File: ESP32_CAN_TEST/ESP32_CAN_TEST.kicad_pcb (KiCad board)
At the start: 2 copper layers, 45.7 x 45.7 mm, 34 parts, among them J1 5V in, J2 Encoder_1, J3 Molex_2x2, J4 Encoder2, J5 i2C, J6 UART, J7 GH1.25, J8 JST_2.54, Q1 2N7002, Q2 2N7002, SW1 EN, SW2 EN, U1 AMS1117, U2 ESP32-WROOM-32, U3 TJA1050

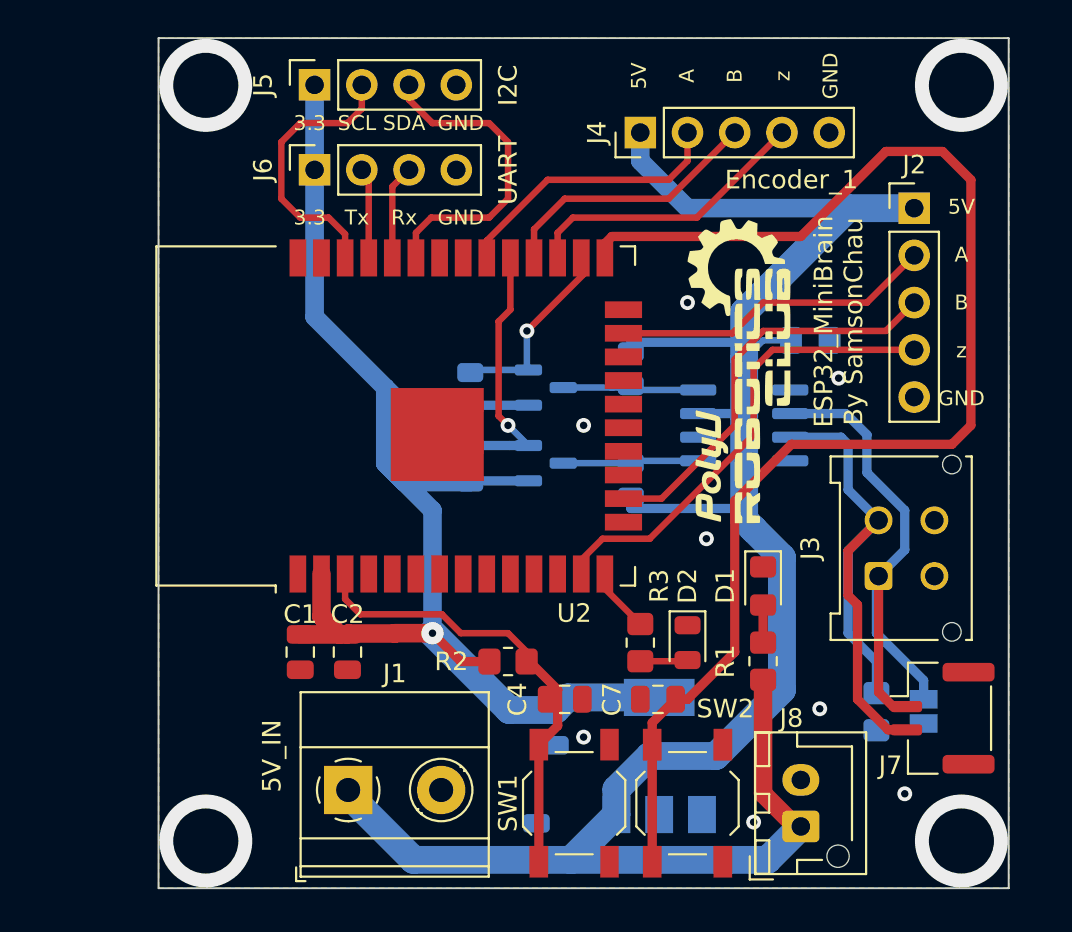
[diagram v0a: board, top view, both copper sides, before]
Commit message: ESP,Power board update
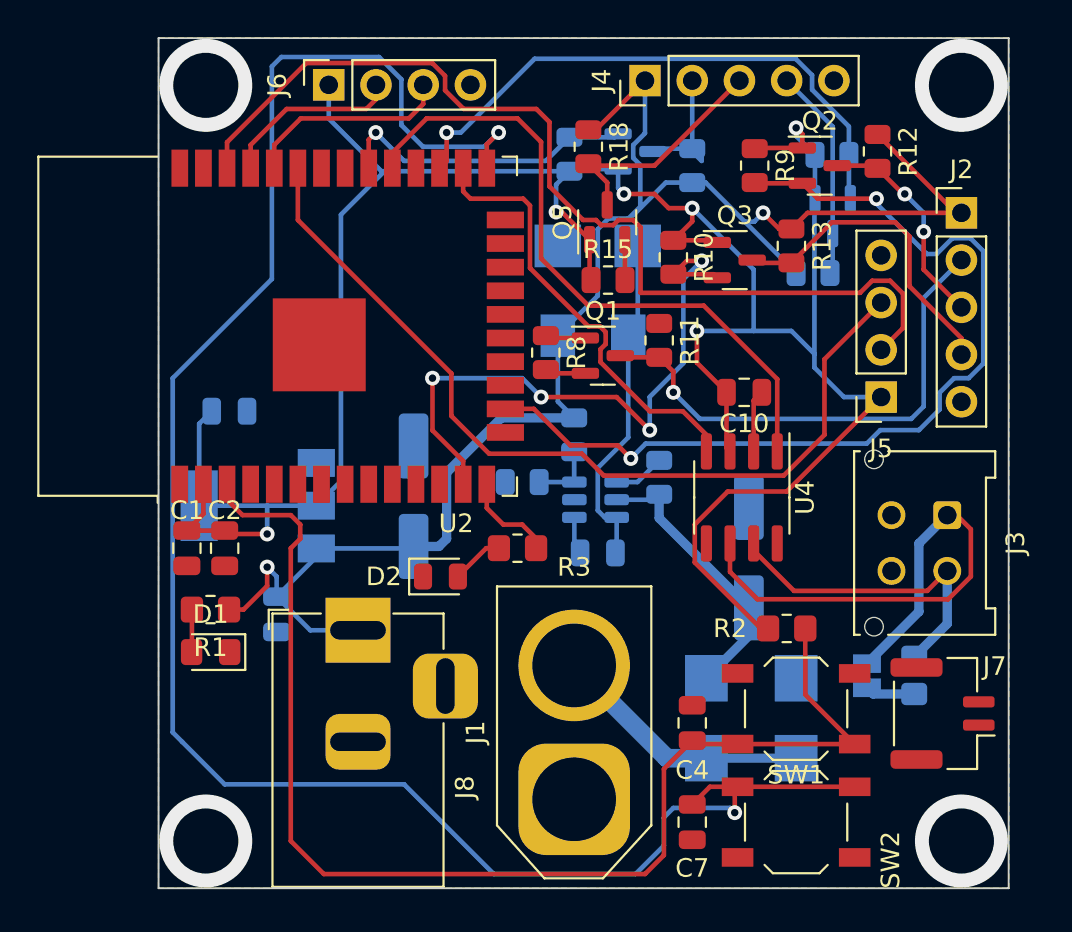
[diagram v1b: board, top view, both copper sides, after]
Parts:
- removed G***: LOGO, PolyuRobotics:Club_logo
- added C10: 0.1u, Capacitor_SMD:C_0805_2012Metric, F.Cu at (133.1, 59.7)
- added C8: 100nF, Capacitor_SMD:C_0805_2012Metric, B.Cu at (125.2, 68.3)
- added C9: 16V 22UF, Capacitor_SMD:CP_Elec_6.3x7.7, B.Cu at (115.3, 65.3)
- added D3: SMBJ24CA, Diode_SMD:D_SMB, B.Cu at (135.9, 77.2)
- added D4: SS34, Diode_SMD:D_SMB, B.Cu at (131.1, 77.2)
- added D5: SS34, Diode_SMD:D_SMB, B.Cu at (125.2, 51.8)
- added L1: 22uH, Inductor_SMD:L_Vishay_IHLP-1616, B.Cu at (125.0, 56.6)
- added Q3: 2N7002, Package_TO_SOT_SMD:SOT-23, F.Cu at (132.6, 52.6)
- added Q4: 2N7002, Package_TO_SOT_SMD:SOT-23, B.Cu at (127.3, 46.7)
- added Q5: 2N7002, Package_TO_SOT_SMD:SOT-23, F.Cu at (125.7, 50.5)
- added Q6: 2N7002, Package_TO_SOT_SMD:SOT-23, B.Cu at (137.9, 50.2)
- added R10: 10K, Resistor_SMD:R_0805_2012Metric, F.Cu at (129.3, 52.4)
- added R11: 10K, Resistor_SMD:R_0805_2012Metric, F.Cu at (128.5, 56.9)
- added R12: 10K, Resistor_SMD:R_0805_2012Metric, F.Cu at (140.3, 46.7)
- added R13: 10K, Resistor_SMD:R_0805_2012Metric, F.Cu at (135.6, 51.8)
- added R14: 10K, Resistor_SMD:R_0805_2012Metric, B.Cu at (123.7, 46.9)
- added R15: 10K, Resistor_SMD:R_0805_2012Metric, F.Cu at (125.8, 53.7)
- added R16: 10K, Resistor_SMD:R_0805_2012Metric, B.Cu at (137.8, 46.9)
- added R17: 10K, Resistor_SMD:R_0805_2012Metric, B.Cu at (130.3, 47.5)
- added R18: 10K, Resistor_SMD:R_0805_2012Metric, F.Cu at (124.7, 46.5)
- added R19: 10K, Resistor_SMD:R_0805_2012Metric, B.Cu at (136.8, 53.3)
- added R9: 10K, Resistor_SMD:R_0805_2012Metric, F.Cu at (133.7, 47.5)
- added U4: SN65HVD230, Package_SO:SOIC-8_3.9x4.9mm_P1.27mm, F.Cu at (133.0, 65.3)
- C6: value 100nF -> 50V 10uF; footprint Capacitor_SMD:C_0805_2012Metric_Pad1.18x1.45mm_HandSolder -> Capacitor_SMD:CP_Elec_6.3x7.7
- J1: value 5V in -> XT60; footprint TerminalBlock_Phoenix:TerminalBlock_Phoenix_MKDS-1,5-2_1x02_P5.00mm_Horizontal -> Connector_AMASS:AMASS_XT60-M_1x02_P7.20mm_Vertical
- J8: value JST_2.54 -> Jack-DC; footprint Connector_JST:JST_XH_B2B-XH-AM_1x02_P2.50mm_Vertical -> Connector_BarrelJack:BarrelJack_Horizontal
- Q1, Q2, R8: moved to F.Cu
- R5: value 10K -> 300K
- R6: value 10K -> 5.1k
- R7: value 10K -> 27K
- U3: value TJA1050 -> AOZ1282CI; footprint Package_SO:SOIC-8_3.9x4.9mm_P1.27mm -> Package_TO_SOT_SMD:SOT-23-6
- moved J5 34.8 mm to (140.5, 59.9), turned to 180 degrees
- moved D1 29.9 mm to (104.4, 73.7), turned to 180 degrees
- moved R1 29.8 mm to (104.4, 71.4), turned to 180 degrees
- moved J8 26.1 mm to (112.3, 72.5)
- moved U1 25.4 mm to (106.9, 65.8), turned to 180 degrees
- moved C5 24.4 mm to (105.4, 60.7), turned to 0 degrees
- moved Q2 19.0 mm to (137.2, 47.5)
- moved C3 18.5 mm to (108.0, 71.6), turned to -90 degrees
- moved R2 15.1 mm to (135.4, 72.4)
- moved D2 13.8 mm to (116.8, 69.6), turned to 0 degrees
- moved SW1 13.0 mm to (135.9, 76.7), turned to 0 degrees
- moved J1 12.2 mm to (124.0, 81.6), turned to 90 degrees
- moved C6 12.1 mm to (133.3, 68.6), turned to 90 degrees
- moved R5 10.2 mm to (128.5, 64.3)
- moved U3 8.94 mm to (125.1, 65.5)
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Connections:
- C6 pad 1: +5V -> Net-(C6-Pad1)
- J1 pad 1: +5V -> GND
- J1 pad 2: GND -> +24V
- J2 pad 2: /IO15 -> Net-(J2-Pad2)
- J2 pad 3: /IO13 -> Net-(J2-Pad3)
- J2 pad 4: /IO14 -> Net-(J2-Pad4)
- J4 pad 2: /IO18 -> Net-(J4-Pad2)
- J4 pad 3: /IO17 -> Net-(J4-Pad3)
- J4 pad 4: /IO16 -> Net-(J4-Pad4)
- J7 pad 1: /CANH+ -> /CANL-
- J7 pad 2: /CANL- -> /CANH+
- Q1 pad 2: /CAN_TX -> /IO15
- Q1 pad 3: Net-(Q1-Pad3) -> Net-(J2-Pad2)
- Q2 pad 2: /CAN_RX -> /IO13
- Q2 pad 3: Net-(Q2-Pad3) -> Net-(J2-Pad3)
- R5 pad 1: +3V3 -> Net-(C6-Pad1)
- R5 pad 2: /CAN_TX -> Net-(R5-Pad2)
- R6 pad 1: +3V3 -> Net-(R6-Pad1)
- R6 pad 2: /CAN_RX -> GND
- R7 pad 1: +5V -> Net-(R6-Pad1)
- R7 pad 2: Net-(Q1-Pad3) -> +5V
- R8 pad 1: +5V -> +3V3
- R8 pad 2: Net-(Q2-Pad3) -> /IO15
- U3 pad 1: Net-(Q1-Pad3) -> Net-(C8-Pad1)
- U3 pad 3: +5V -> Net-(R6-Pad1)
- U3 pad 4: Net-(Q2-Pad3) -> Net-(R5-Pad2)
- U3 pad 5: unconnected-(U3-Pad5) -> Net-(C6-Pad1)
- U3 pad 6: /CANH+ -> Net-(C8-Pad2)
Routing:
- net +3V3: track 77.1 -> 141.5 mm, vias 1 -> 6
- net Net-(C4-Pad1): track 24.8 -> 66.7 mm
- net /SCL: track 14.9 -> 53.5 mm
- net Net-(C7-Pad2): track 72.4 -> 102.8 mm, vias 0 -> 2
- net +5V: track 119.3 -> 89.0 mm, vias 0 -> 2
- net /SDA: track 17.2 -> 47.4 mm
- net /IO13: track 22.1 -> 50.2 mm, vias 0 -> 2
- net Net-(J2-Pad2): track 0.00 -> 27.4 mm, vias 0 -> 1
- net /CAN_TX: track 14.2 -> 35.7 mm, vias 1 -> 0
- net Net-(C8-Pad2): track 0.00 -> 18.2 mm
- net Net-(J2-Pad4): track 0.00 -> 17.2 mm
- net /IO16: track 15.6 -> 31.2 mm, vias 0 -> 1
- net Net-(C6-Pad1): track 0.00 -> 15.2 mm
- net /IO15: track 17.4 -> 2.21 mm
- net /CANL-: track 32.5 -> 17.5 mm
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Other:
- board text removed: "3.3"
- board text removed: "5V"
- board text removed: "5V A B z GND"
- board text removed: "5V_IN"
- board text removed: "ESP32_MiniBrain By SamsonChau"
- board text removed: "Encoder_1"
- board text removed: "GND"
- board text removed: "I2C"
- board text removed: "Rx"
- board text removed: "SCL"
- board text removed: "SDA"
- board text removed: "Tx"
- board text removed: "UART"
